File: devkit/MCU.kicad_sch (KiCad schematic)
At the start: 41 parts, among them IC601 FAN5622SX, IC602 USBLC6-2P6, IC603 MX25U51245GZ4I00, IC604 NTS0104GU12, J601 Jumper, J602 Jumper, J603 Jumper, J604 Jumper, M601 NORA-B106, X601 DEBUG, X602 Current, X603 Device, X604 UART, X605 GPIO, X606 Current, X607 IO Current, X608 Display, X609 Current, X610 LED Current

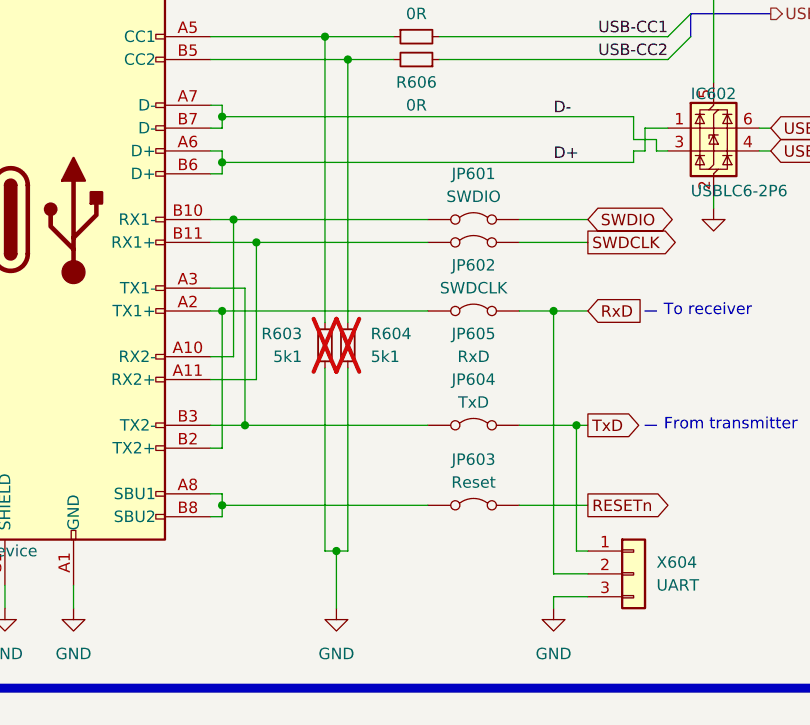
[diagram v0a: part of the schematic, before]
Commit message: Revert "Task: Issue #173"
This reverts commit e04384c88487c0ad4268dbede6dd77cc14cfed5f.
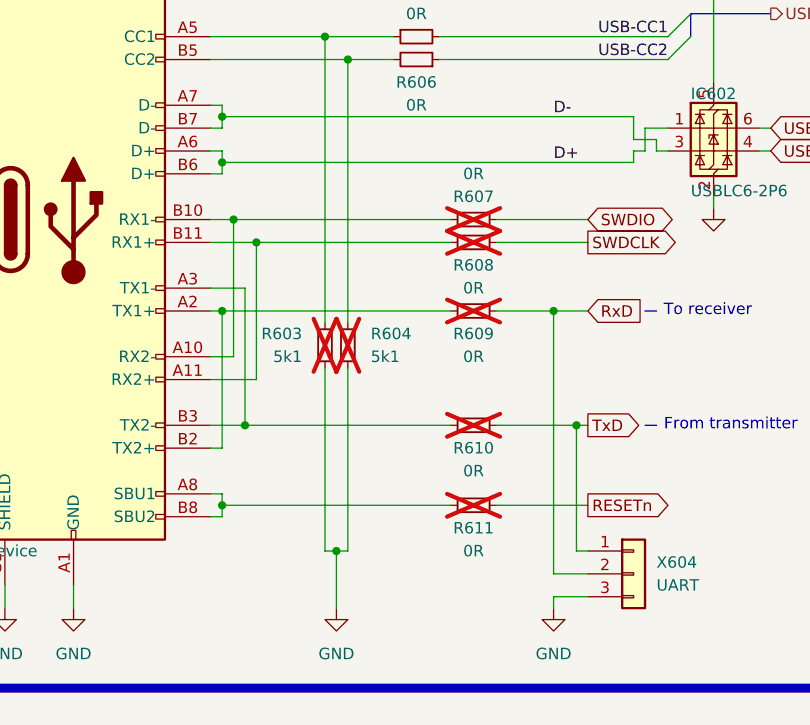
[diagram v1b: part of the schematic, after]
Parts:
- removed JP601: SWDIO, Jumper:SolderJumper-2_P1.3mm_Bridged_RoundedPad1.0x1.5mm, symbol Jumper:Jumper_2_Bridged
- removed JP602: SWDCLK, Jumper:SolderJumper-2_P1.3mm_Bridged_RoundedPad1.0x1.5mm, symbol Jumper:Jumper_2_Bridged
- removed JP603: Reset, Jumper:SolderJumper-2_P1.3mm_Bridged_RoundedPad1.0x1.5mm, symbol Jumper:Jumper_2_Bridged
- removed JP604: TxD, Jumper:SolderJumper-2_P1.3mm_Bridged_RoundedPad1.0x1.5mm, symbol Jumper:Jumper_2_Bridged
- removed JP605: RxD, Jumper:SolderJumper-2_P1.3mm_Bridged_RoundedPad1.0x1.5mm, symbol Jumper:Jumper_2_Bridged
- added R607, R608, R609, R610, R611: 0R, Resistor_SMD:R_0805_2012Metric, symbol Device:R_Small
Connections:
- net RESETn: now also R611.1
- net RxD: now also R609.1
- net SWDCLK: now also R608.1
- net SWDIO: now also R607.1
- net TxD: now also R610.1
- net at X603.A8 (SBU1), X603.B8 (SBU2): now also R611.2
- net at X603.A2 (TX1+), X603.B2 (TX2+): now also R609.2
- net at X603.A10 (RX2-), X603.B10 (RX1-): now also R607.2
- net at X603.A11 (RX2+), X603.B11 (RX1+): now also R608.2
- net at X603.A3 (TX1-), X603.B3 (TX2-): now also R610.2
